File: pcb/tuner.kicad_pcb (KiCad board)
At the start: 2 copper layers, 120.8 x 69.8 mm, 14 parts, among them J1 RN112BPC, SW1 SW_Push, SW4 SW_Push, U1 XIAO-nRF52840-SMD, U2 09816, U3 Adafruit LiIon/LiPoly Backpack

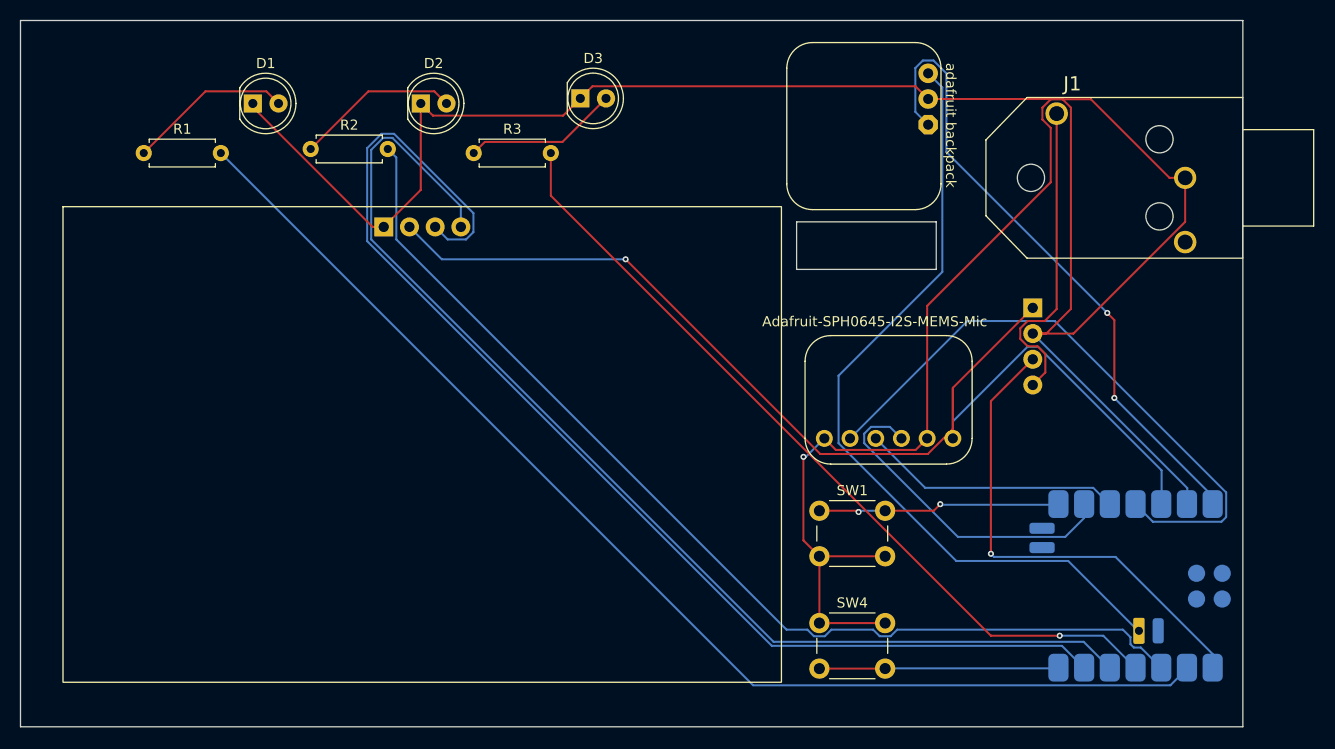
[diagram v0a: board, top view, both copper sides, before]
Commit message: Add files via upload
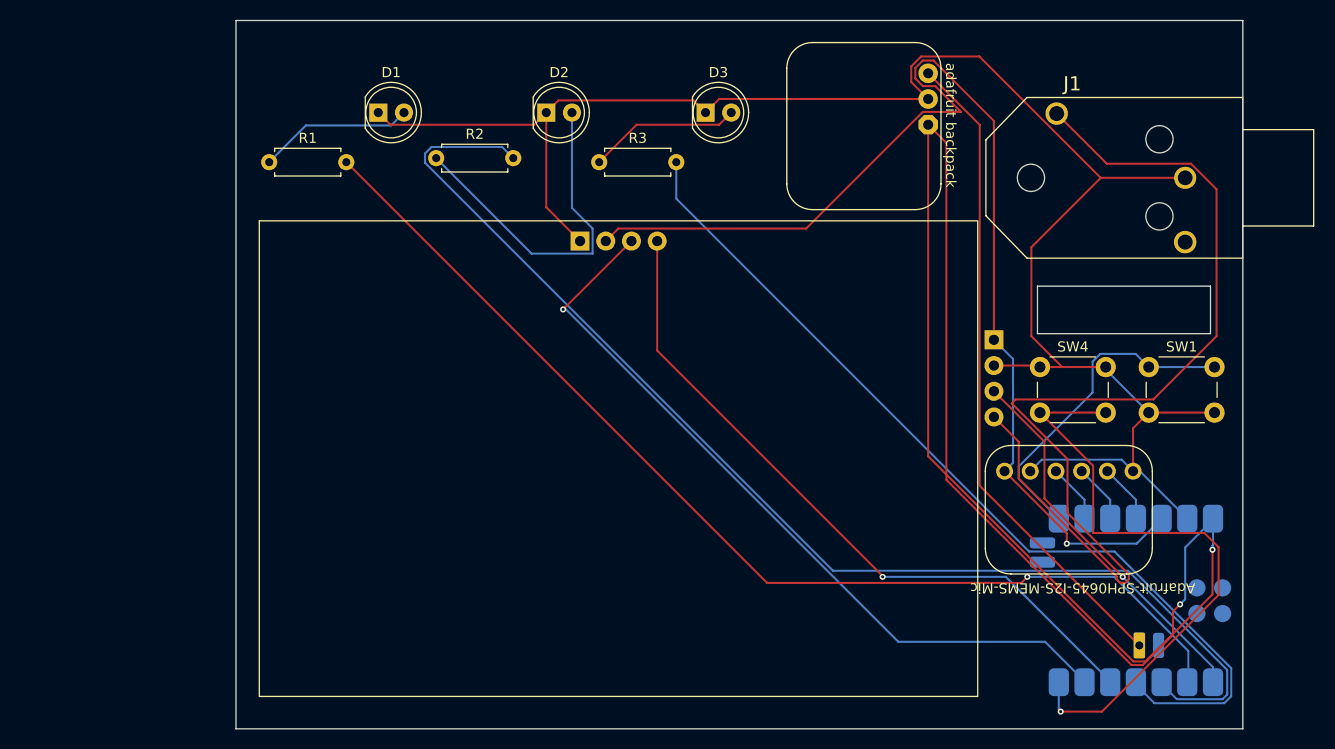
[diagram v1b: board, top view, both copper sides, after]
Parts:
- moved SW1 35.5 mm to (149.1, 108.2)
- moved SW4 33.4 mm to (138.3, 108.2)
- moved MIC1 21.0 mm to (141.2, 122.4), turned to 180 degrees
- moved OL1 19.5 mm to (96.7, 117.2)
- moved D3 12.5 mm to (105.3, 83.0)
- moved D2 12.4 mm to (89.6, 83.0)
- moved R2 12.4 mm to (78.7, 87.5)
- moved R3 12.4 mm to (94.8, 87.9)
- moved R1 12.4 mm to (62.2, 87.9)
- moved D1 12.4 mm to (73.0, 83.0)
- moved U2 4.97 mm to (126.8, 109.0)
- moved U1 1.44 mm to (147.9, 131.3)
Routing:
- net +5V: track 63.5 -> 159.7 mm
- net GND: track 270.4 -> 178.8 mm, vias 1 -> 0
- net Net-(U2-IN): track 31.4 -> 101.2 mm
- net Net-(MIC1-WS): track 61.2 -> 5.86 mm
- net Net-(OL1-SDA): track 113.6 -> 69.3 mm, vias 0 -> 1
- net Net-(OL1-SCL): track 118.4 -> 76.6 mm, vias 0 -> 1
- net Net-(U1-P1.11_D6_TX): track 23.7 -> 61.6 mm, vias 0 -> 1
- net Net-(MIC1-CLK): track 33.1 -> 5.86 mm
- net Net-(MIC1-DAT): track 25.9 -> 5.86 mm
- net Net-(D2-A): track 16.3 -> 34.2 mm
- net Net-(U1-P0.28_A2_D2): track 104.0 -> 120.2 mm
- net BAT: track 78.8 -> 65.2 mm
- net Net-(U1-P0.03_A1_D1): track 118.0 -> 106.8 mm, vias 0 -> 1
- net Net-(U1-P0.02_A0_D0): track 48.4 -> 37.7 mm
- net Net-(U1-P0.29_A3_D3): track 81.4 -> 91.1 mm, vias 1 -> 0
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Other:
- board size 120.8 x 69.8 mm -> 99.5 x 70 mm
